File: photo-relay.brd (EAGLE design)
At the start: 45 x 45 mm, 12 parts, among them IC1 LM393N, K1 G5L, T1 2N3904, X1 MKDSN1,5/3-5,08, X2 MKDSN1,5/2-5,08

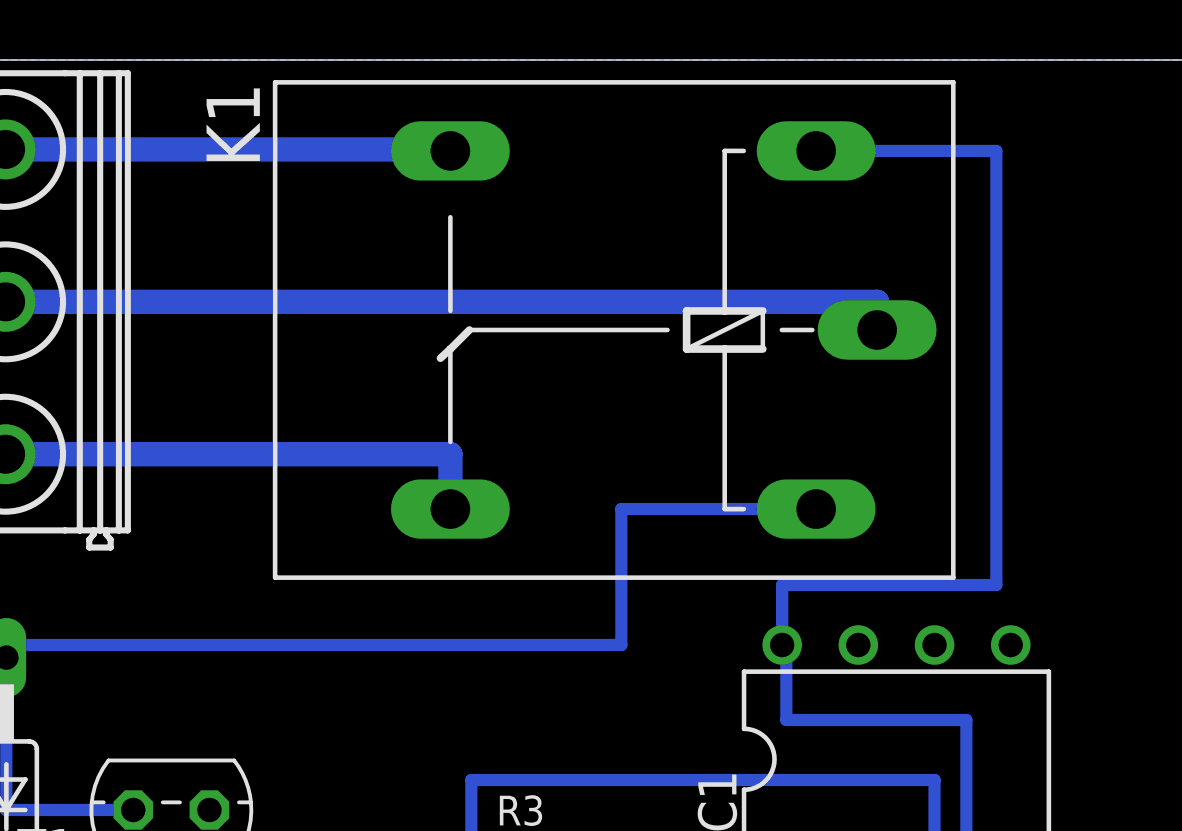
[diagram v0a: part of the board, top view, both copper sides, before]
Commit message: minor fix.
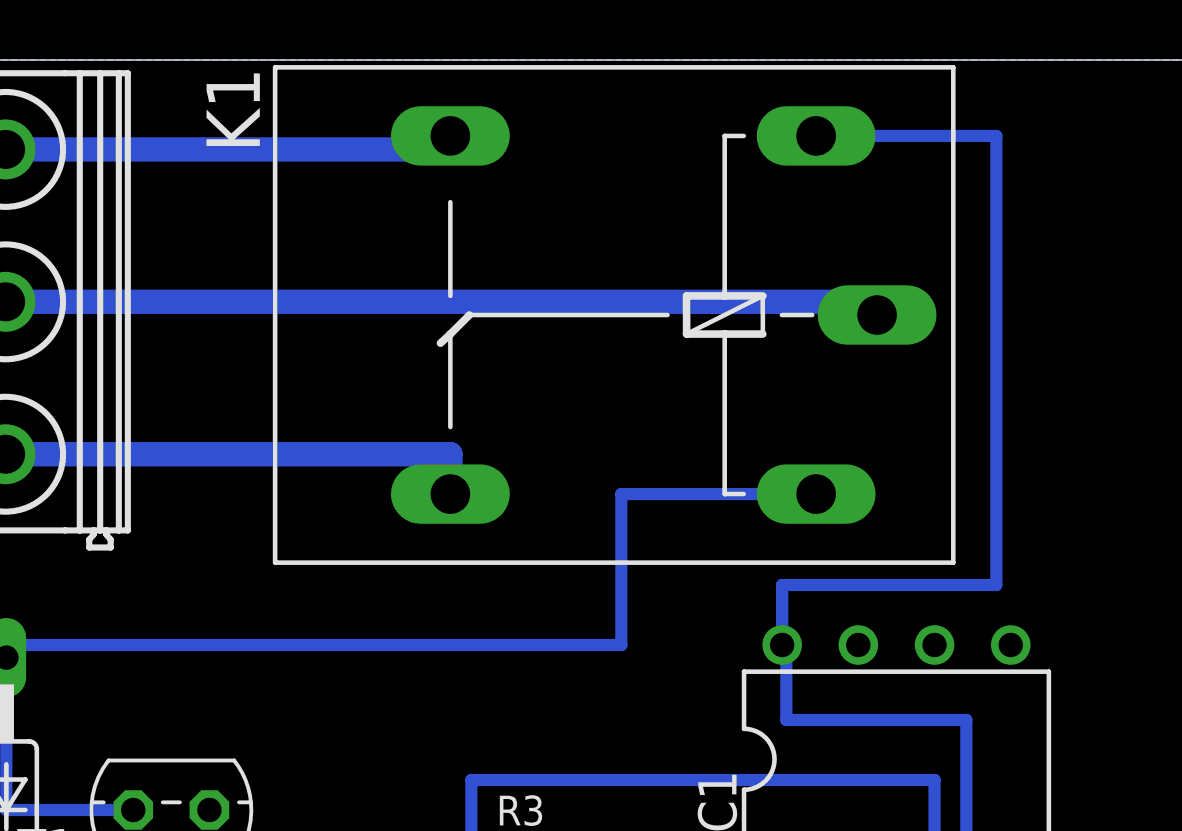
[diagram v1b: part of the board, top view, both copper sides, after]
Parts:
- moved K1 0.50 mm to (23.5, 36.5)
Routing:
- net V+: track 114.3 -> 114.8 mm
- net N$9: track 16.7 -> 16.2 mm
- net N$7: track 41.3 -> 41.8 mm
- net N$5: track 30.0 -> 29.5 mm
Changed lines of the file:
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@@
 <grid distance="0.5" unitdist="mm" unit="mm" style="lines" multiple="1" display="yes" altdistance="0.025" altunitdist="inch" altunit="inch"/>
 <layers>
-<layer number="1" name="Top" color="4" fill="1" visible="no" active="yes"/>
+<layer number="1" name="Top" color="4" fill="1" visible="yes" active="yes"/>
 <layer number="16" name="Bottom" color="1" fill="1" visible="yes" active="yes"/>
 <layer number="17" name="Pads" color="2" fill="1" visible="yes" active="yes"/>
 <layer number="18" name="Vias" color="2" fill="1" visible="yes" active="yes"/>
-<layer number="19" name="Unrouted" color="6" fill="1" visible="no" active="yes"/>
+<layer number="19" name="Unrouted" color="6" fill="1" visible="yes" active="yes"/>
 <layer number="20" name="Dimension" color="15" fill="1" visible="yes" active="yes"/>
-<layer number="21" name="tPlace" color="7" fill="1" visible="no" active="yes"/>
-<layer number="22" name="bPlace" color="7" fill="1" visible="no" active="yes"/>
-<layer number="23" name="tOrigins" color="15" fill="1" visible="no" active="yes"/>
-<layer number="24" name="bOrigins" color="15" fill="1" visible="no" active="yes"/>
-<layer number="25" name="tNames" color="7" fill="1" visible="no" active="yes"/>
-<layer number="26" name="bNames" color="7" fill="1" visible="no" active="yes"/>
-<layer number="27" name="tValues" color="7" fill="1" visible="no" active="yes"/>
-<layer number="28" name="bValues" color="7" fill="1" visible="no" active="yes"/>
-<layer number="29" name="tStop" color="7" fill="3" visible="no" active="yes"/>
-<layer number="30" name="bStop" color="7" fill="6" visible="no" active="yes"/>
-<layer number="31" name="tCream" color="7" fill="4" visible="no" active="yes"/>
-<layer number="32" name="bCream" color="7" fill="5" visible="no" active="yes"/>
-<layer number="33" name="tFinish" color="6" fill="3" visible="no" active="yes"/>
-<layer number="34" name="bFinish" color="6" fill="6" visible="no" active="yes"/>
-<layer number="35" name="tGlue" color="7" fill="4" visible="no" active="yes"/>
-<layer number="36" name="bGlue" color="7" fill="5" visible="no" active="yes"/>
-<layer number="37" name="tTest" color="7" fill="1" visible="no" active="yes"/>
-<layer number="38" name="bTest" color="7" fill="1" visible="no" active="yes"/>
-<layer number="39" name="tKeepout" color="4" fill="11" visible="no" active="yes"/>
-<layer number="40" name="bKeepout" color="1" fill="11" visible="no" active="yes"/>
-<layer number="41" name="tRestrict" color="4" fill="10" visible="no" active="yes"/>
-<layer number="42" name="bRestrict" color="1" fill="10" visible="no" active="yes"/>
-<layer number="43" name="vRestrict" color="2" fill="10" visible="no" active="yes"/>
-<layer number="44" name="Drills" color="7" fill="1" visible="no" active="yes"/>
-<layer number="45" name="Holes" color="7" fill="1" visible="no" active="yes"/>
-<layer number="46" name="Milling" color="3" fill="1" visible="no" active="yes"/>
-<layer number="47" name="Measures" color="7" fill="1" visible="no" active="yes"/>
-<layer number="48" name="Document" color="7" fill="1" visible="no" active="yes"/>
-<layer number="49" name="Reference" color="7" fill="1" visible="no" active="yes"/>
-<layer number="51" name="tDocu" color="7" fill="1" visible="no" active="yes"/>
-<layer number="52" name="bDocu" color="7" fill="1" visible="no" active="yes"/>
+<layer number="21" name="tPlace" color="7" fill="1" visible="yes" active="yes"/>
+<layer number="22" name="bPlace" color="7" fill="1" visible="yes" active="yes"/>
+<layer number="23" name="tOrigins" color="15" fill="1" visible="yes" active="yes"/>
+<layer number="24" name="bOrigins" color="15" fill="1" visible="yes" active="yes"/>
+<layer number="25" name="tNames" color="7" fill="1" visible="yes" active="yes"/>
+<layer number="26" name="bNames" color="7" fill="1" visible="yes" active="yes"/>
+<layer number="27" name="tValues" color="7" fill="1" visible="yes" active="yes"/>
+<layer number="28" name="bValues" color="7" fill="1" visible="yes" active="yes"/>
+<layer number="29" name="tStop" color="7" fill="3" visible="yes" active="yes"/>
+<layer number="30" name="bStop" color="7" fill="6" visible="yes" active="yes"/>
+<layer number="31" name="tCream" color="7" fill="4" visible="yes" active="yes"/>
+<layer number="32" name="bCream" color="7" fill="5" visible="yes" active="yes"/>
+<layer number="33" name="tFinish" color="6" fill="3" visible="yes" active="yes"/>
+<layer number="34" name="bFinish" color="6" fill="6" visible="yes" active="yes"/>
+<layer number="35" name="tGlue" color="7" fill="4" visible="yes" active="yes"/>
+<layer number="36" name="bGlue" color="7" fill="5" visible="yes" active="yes"/>
+<layer number="37" name="tTest" color="7" fill="1" visible="yes" active="yes"/>
+<layer number="38" name="bTest" color="7" fill="1" visible="yes" active="yes"/>
+<layer number="39" name="tKeepout" color="4" fill="11" visible="yes" active="yes"/>
+<layer number="40" name="bKeepout" color="1" fill="11" visible="yes" active="yes"/>
+<layer number="41" name="tRestrict" color="4" fill="10" visible="yes" active="yes"/>
+<layer number="42" name="bRestrict" color="1" fill="10" visible="yes" active="yes"/>
+<layer number="43" name="vRestrict" color="2" fill="10" visible="yes" active="yes"/>
+<layer number="44" name="Drills" color="7" fill="1" visible="yes" active="yes"/>
+<layer number="45" name="Holes" color="7" fill="1" visible="yes" active="yes"/>
+<layer number="46" name="Milling" color="3" fill="1" visible="yes" active="yes"/>
+<layer number="47" name="Measures" color="7" fill="1" visible="yes" active="yes"/>
+<layer number="48" name="Document" color="7" fill="1" visible="yes" active="yes"/>
+<layer number="49" name="Reference" color="7" fill="1" visible="yes" active="yes"/>
+<layer number="51" name="tDocu" color="7" fill="1" visible="yes" active="yes"/>
+<layer number="52" name="bDocu" color="7" fill="1" visible="yes" active="yes"/>
 <layer number="90" name="Modules" color="5" fill="1" visible="no" active="no"/>
 <layer number="91" name="Nets" color="2" fill="1" visible="no" active="no"/>
@@
 <element name="D1" library="diode" package="DO35-10" value="1N4148DO35-10" x="4" y="20" rot="R90"/>
 <element name="T1" library="transistor" package="TO92" value="2N3904" x="9.5" y="20" rot="R180"/>
-<element name="K1" library="relay" package="G5LE" value="G5L" x="23.5" y="36" rot="R180">
-<attribute name="MF" value="" x="23.5" y="36" size="1.778" layer="27" rot="R180" display="off"/>
-<attribute name="OC_NEWARK" value="unknown" x="23.5" y="36" size="1.778" layer="27" rot="R180" display="off"/>
-<attribute name="MPN" value="" x="23.5" y="36" size="1.778" layer="27" rot="R180" display="off"/>
-<attribute name="OC_FARNELL" value="unknown" x="23.5" y="36" size="1.778" layer="27" rot="R180" display="off"/>
+<element name="K1" library="relay" package="G5LE" value="G5L" x="23.5" y="36.5" rot="R180">
+<attribute name="MF" value="" x="23.5" y="36.5" size="1.778" layer="27" rot="R180" display="off"/>
+<attribute name="OC_NEWARK" value="unknown" x="23.5" y="36.5" size="1.778" layer="27" rot="R180" display="off"/>
+<attribute name="MPN" value="" x="23.5" y="36.5" size="1.778" layer="27" rot="R180" display="off"/>
+<attribute name="OC_FARNELL" value="unknown" x="23.5" y="36.5" size="1.778" layer="27" rot="R180" display="off"/>
 </element>
 </elements>
@@
 <wire x1="9.69" y1="14.92" x2="9.69" y2="15" width="0.4064" layer="16"/>
 <contactref element="K1" pad="1"/>
-<wire x1="30.993" y1="41.969" x2="37" y2="41.969" width="0.4064" layer="16"/>
-<wire x1="37" y1="41.969" x2="37" y2="27.5" width="0.4064" layer="16"/>
+<wire x1="30.993" y1="42.469" x2="37" y2="42.469" width="0.4064" layer="16"/>
+<wire x1="37" y1="42.469" x2="37" y2="27.5" width="0.4064" layer="16"/>
 <wire x1="37" y1="27.5" x2="29.86" y2="27.5" width="0.4064" layer="16"/>
 <wire x1="29.86" y1="27.5" x2="29.86" y2="25.5" width="0.4064" layer="16"/>
@@
 <contactref element="X2" pad="1"/>
 <contactref element="T1" pad="3"/>
-<wire x1="12.03" y1="6.82" x2="10.77" y2="20" width="0" layer="19" extent="1-1"/>
 </signal>
 <signal name="N$6">
@@
 <wire x1="8.23" y1="20" x2="4" y2="20" width="0.4064" layer="16"/>
 <contactref element="K1" pad="2"/>
-<wire x1="30.993" y1="30.031" x2="24.5" y2="30.031" width="0.4064" layer="16"/>
-<wire x1="24.5" y1="30.031" x2="24.5" y2="25.5" width="0.4064" layer="16"/>
+<wire x1="30.993" y1="30.531" x2="24.5" y2="30.531" width="0.4064" layer="16"/>
+<wire x1="24.5" y1="30.531" x2="24.5" y2="25.5" width="0.4064" layer="16"/>
 <wire x1="24.5" y1="25.5" x2="4" y2="25.5" width="0.4064" layer="16"/>
 <wire x1="4" y1="25.5" x2="4" y2="25.08" width="0.4064" layer="16"/>
@@
 <contactref element="X1" pad="2"/>
 <wire x1="3.975" y1="36.9389" x2="33.025" y2="36.9389" width="0.8128" layer="16"/>
-<wire x1="33.025" y1="36.9389" x2="33.025" y2="36" width="0.8128" layer="16"/>
+<wire x1="33.025" y1="36.9389" x2="33.025" y2="36.5" width="0.8128" layer="16"/>
 </signal>
 <signal name="N$8">
@@
 <contactref element="X1" pad="3"/>
 <wire x1="3.975" y1="42.0189" x2="18.801" y2="42.0189" width="0.8128" layer="16"/>
-<wire x1="18.801" y1="42.0189" x2="18.801" y2="41.969" width="0.8128" layer="16"/>
+<wire x1="18.801" y1="42.0189" x2="18.801" y2="42.469" width="0.8128" layer="16"/>
 </signal>
 <signal name="N$9">
@@
 <contactref element="K1" pad="O"/>
 <wire x1="3.975" y1="31.8589" x2="18.801" y2="31.8589" width="0.8128" layer="16"/>
-<wire x1="18.801" y1="31.8589" x2="18.801" y2="30.031" width="0.8128" layer="16"/>
+<wire x1="18.801" y1="31.8589" x2="18.801" y2="30.531" width="0.8128" layer="16"/>
 </signal>
 </signals>
